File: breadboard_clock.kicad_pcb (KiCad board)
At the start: 2 copper layers, 54 x 53.5 mm, 42 parts, among them J1 Conn_01x02_Male, J2 Conn_01x03_Male, J3 USB_C_Receptacle_USB2.0, P1 1M, SW1 SW_Push, SW2 SW_SPDT, U1 ICM7555, U2 74LS04-Full, U3 74LS08-Full, U5 ICM7555, U8 ICM7555

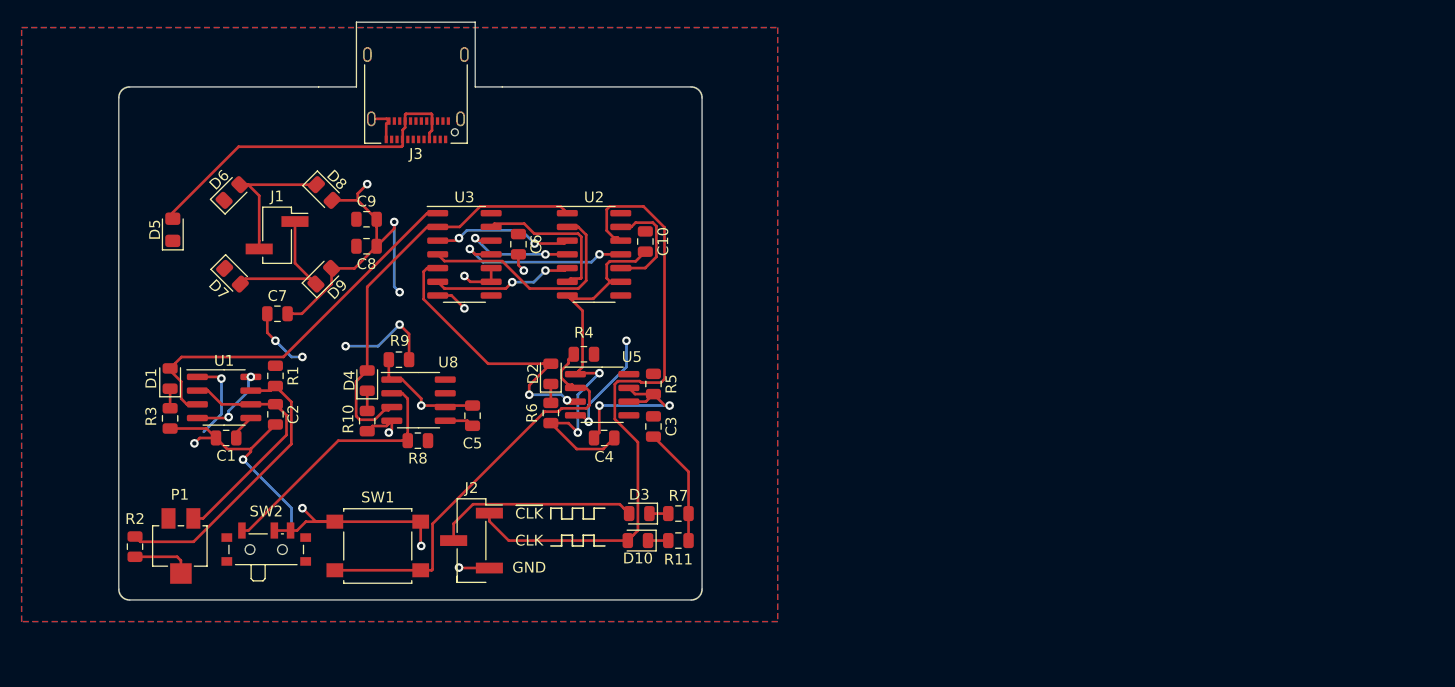
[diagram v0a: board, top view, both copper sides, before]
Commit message: Add files via upload
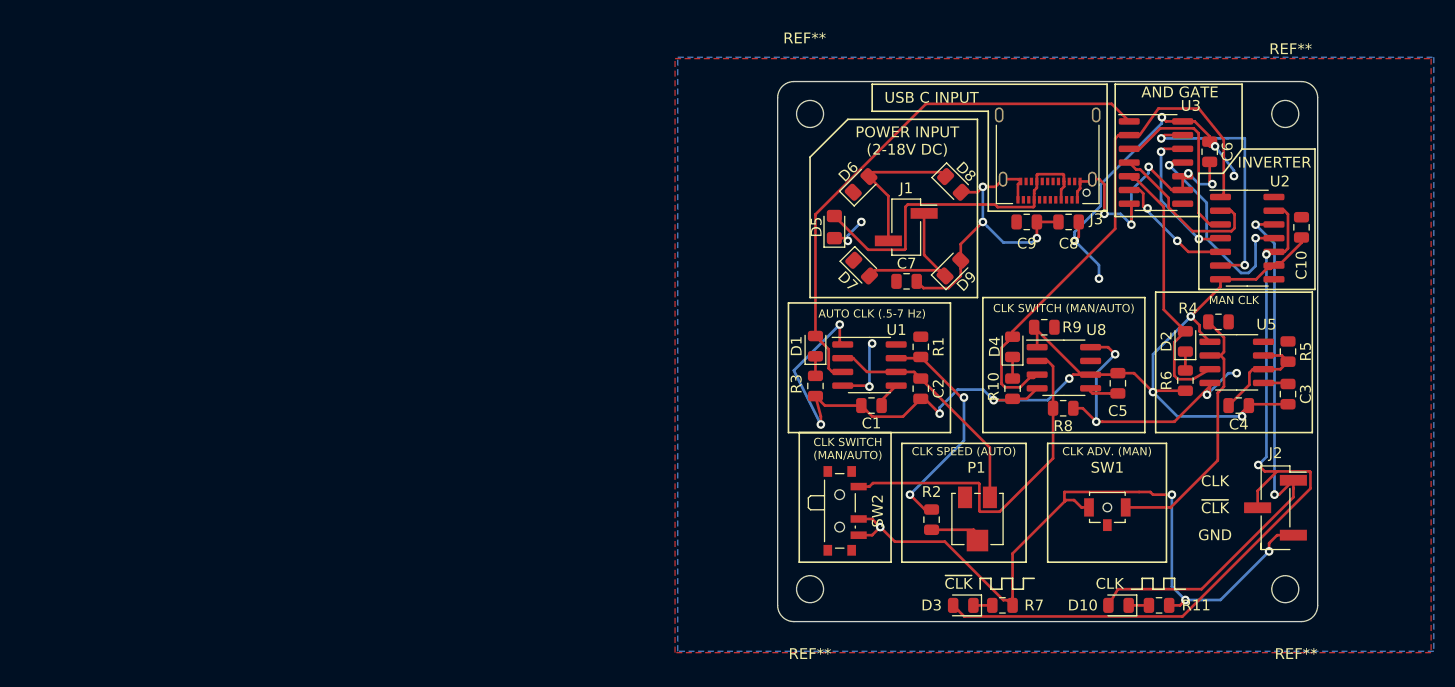
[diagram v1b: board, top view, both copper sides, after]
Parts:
- added G***: LOGO, breadboard_clock-master:github_image, B.Cu at (467.5, 80.0)
- added REF**: MountingHole_2.5mm, MountingHole:MountingHole_2.5mm, F.Cu at (222.0, 78.0)
- added REF**: MountingHole_2.5mm, MountingHole:MountingHole_2.5mm, F.Cu at (222.0, 122.0)
- added REF**: MountingHole_2.5mm, MountingHole:MountingHole_2.5mm, F.Cu at (178.0, 122.0)
- added REF**: MountingHole_2.5mm, MountingHole:MountingHole_2.5mm, F.Cu at (178.0, 78.0)
- P1: footprint Potentiometer_SMD:Potentiometer_Bourns_3224X_Vertical -> Potentiometer_SMD:Potentiometer_Bourns_3314J_Vertical
- SW1: footprint Button_Switch_SMD:SW_SPST_B3S-1000 -> Button_Switch_SMD:SW_SPST_B3U-1100P-B
- moved J2 74.5 mm to (221.1, 114.5)
- moved P1 73.8 mm to (193.5, 115.5)
- moved R2 73.8 mm to (189.2, 115.6)
- moved SW1 67.6 mm to (205.5, 115.2)
- moved C8 65.0 mm to (201.9, 88.0), turned to 0 degrees
- moved U3 64.6 mm to (210.0, 82.5)
- moved C6 64.6 mm to (215.0, 81.5)
- moved D5 61.3 mm to (180.2, 88.5)
- moved C9 61.1 mm to (198.1, 88.0)
- moved C10 60.8 mm to (223.5, 88.5)
- moved U2 60.5 mm to (218.5, 89.5)
- moved D4 59.8 mm to (196.8, 99.6)
- moved C1 59.8 mm to (183.7, 105.0)
- moved C5 59.8 mm to (206.5, 102.9)
- moved D1 59.8 mm to (178.5, 99.5)
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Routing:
- net GND: track 160.8 -> 239.1 mm, vias 16 -> 20
- net CLK: track 29.1 -> 75.8 mm, vias 0 -> 2
- net VCC: track 33.3 -> 70.4 mm, vias 8 -> 13
- net Net-(D1-Pad2): track 35.9 -> 50.2 mm
- net Net-(R4-Pad2): track 39.5 -> 25.2 mm
- net Net-(D4-Pad2): track 38.2 -> 49.3 mm
- net Net-(U2-Pad6): track 14.2 -> 23.9 mm, vias 0 -> 2
- net Net-(R8-Pad2): track 24.4 -> 33.0 mm
- net Net-(C4-Pad1): track 16.7 -> 10.3 mm, vias 2 -> 0
- net ~CLK: track 58.9 -> 52.8 mm, vias 0 -> 2
- net Net-(U2-Pad2): track 21.7 -> 15.7 mm
- net Net-(R1-Pad2): track 26.9 -> 21.5 mm, vias 0 -> 2
- net Net-(U2-Pad3): track 13.0 -> 17.2 mm, vias 2 -> 0
- net Net-(U2-Pad11): track 17.0 -> 20.0 mm
- net Net-(U2-Pad4): track 10.7 -> 13.7 mm
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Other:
- board size 54 x 53.5 mm -> 50 x 50 mm
- board text added: "555 TIMER CLOCK DESIGNED BY b0xmaker github.com/b0xmaker/breadboard_clock v0: PCB CREATED 2021-06-20"
- board text added: "AND GATE"
- board text added: "AUTO CLK (.5-7 Hz)"
- board text added: "CLK ADV. (MAN)"
- board text added: "CLK SPEED (AUTO)"
- board text added: "CLK SWITCH (MAN/AUTO)"
- board text added: "INVERTER"
- board text added: "MAN CLK"
- board text added: "POWER INPUT (2-18V DC)"
- board text added: "USB C INPUT"
